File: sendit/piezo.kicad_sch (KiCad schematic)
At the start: 3 parts, among them Q4 AO3400A

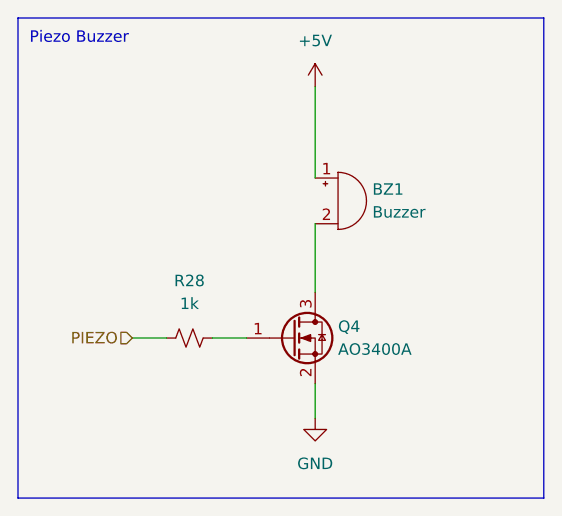
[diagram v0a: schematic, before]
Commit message: piezo resistor
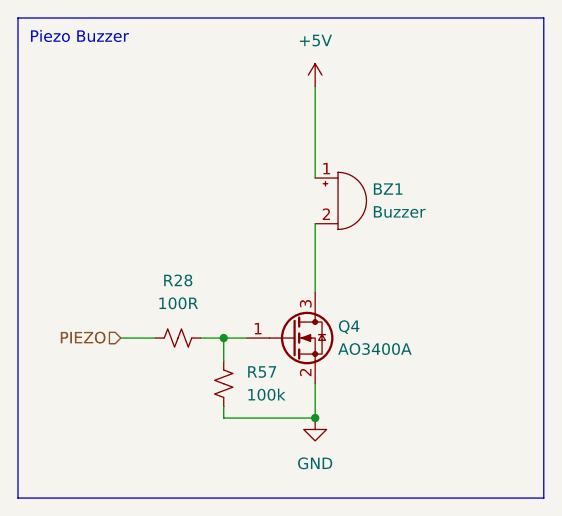
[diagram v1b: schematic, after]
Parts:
- added R57: 100k, Resistor_SMD:R_0603_1608Metric, symbol Device:R_Small_US
- R28: value 1k -> 100R; LCSC C95781 -> (none)
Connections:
- net GND: now also R57.2
- net at Q4.1 (G), R28.1: now also R57.1
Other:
- moved on the sheet: R28
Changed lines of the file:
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@@
 		)
+	)
+	(junction
+		(at 143.51 102.87)
+		(diameter 0)
+		(color 0 0 0 0)
+	)
+	(junction
+		(at 133.35 93.98)
+		(diameter 0)
+		(color 0 0 0 0)
 	)
 	(wire
@@
 	(wire
 		(pts
+			(xy 133.35 93.98) (xy 135.89 93.98)
+		)
+		(stroke
+			(width 0)
+			(type default)
+		)
+	)
+	(wire
+		(pts
+			(xy 133.35 93.98) (xy 133.35 96.52)
+		)
+		(stroke
+			(width 0)
+			(type default)
+		)
+	)
+	(wire
+		(pts
 			(xy 143.51 66.04) (xy 143.51 76.2)
 		)
@@
 	(wire
 		(pts
-			(xy 132.08 93.98) (xy 135.89 93.98)
+			(xy 130.81 93.98) (xy 133.35 93.98)
 		)
 		(stroke
@@
 	(wire
 		(pts
-			(xy 123.19 93.98) (xy 127 93.98)
+			(xy 133.35 101.6) (xy 133.35 102.87)
+		)
+		(stroke
+			(width 0)
+			(type default)
+		)
+	)
+	(wire
+		(pts
+			(xy 121.92 93.98) (xy 125.73 93.98)
+		)
+		(stroke
+			(width 0)
+			(type default)
+		)
+	)
+	(wire
+		(pts
+			(xy 133.35 102.87) (xy 143.51 102.87)
 		)
 		(stroke
@@
 	(hierarchical_label "PIEZO"
 		(shape input)
-		(at 123.19 93.98 180)
+		(at 121.92 93.98 180)
 		(effects
 			(font
@@
 	(symbol
 		(lib_id "Device:R_Small_US")
-		(at 129.54 93.98 270)
+		(at 128.27 93.98 270)
 		(unit 1)
 		(exclude_from_sim no)
@@
 		(fields_autoplaced yes)
 		(property "Reference" "R28"
-			(at 129.54 87.63 90)
-			(effects
-				(font
-					(size 1.27 1.27)
-				)
-			)
-		)
-		(property "Value" "1k"
-			(at 129.54 90.17 90)
+			(at 128.27 87.63 90)
+			(effects
+				(font
+					(size 1.27 1.27)
+				)
+			)
+		)
+		(property "Value" "100R"
+			(at 128.27 90.17 90)
 			(effects
 				(font
@@
 		)
 		(property "Footprint" "Resistor_SMD:R_0603_1608Metric"
-			(at 129.54 93.98 0)
+			(at 128.27 93.98 0)
 			(effects
 				(font
@@
 		)
 		(property "Datasheet" "~"
-			(at 129.54 93.98 0)
+			(at 128.27 93.98 0)
 			(effects
 				(font
@@
 		)
 		(property "Description" "Resistor, small US symbol"
-			(at 129.54 93.98 0)
-			(effects
-				(font
-					(size 1.27 1.27)
-				)
-				(hide yes)
-			)
-		)
-		(property "LCSC" "C95781"
-			(at 129.54 93.98 0)
-			(effects
-				(font
-					(size 1.27 1.27)
-				)
-				(hide yes)
-			)
-		)
-		(property "ALT" ""
-			(at 129.54 93.98 0)
+			(at 128.27 93.98 0)
 			(effects
 				(font
@@
 					(unit 1)
 				)
+			)
+		)
+	)
+	(symbol
+		(lib_id "Device:R_Small_US")
+		(at 133.35 99.06 0)
+		(unit 1)
+		(exclude_from_sim no)
+		(in_bom yes)
+		(on_board yes)
+		(dnp no)
+		(fields_autoplaced yes)
+		(property "Reference" "R57"
+			(at 135.89 97.7899 0)
+			(effects
+				(font
+					(size 1.27 1.27)
+				)
+				(justify left)
+			)
+		)
+		(property "Value" "100k"
+			(at 135.89 100.3299 0)
+			(effects
+				(font
+					(size 1.27 1.27)
+				)
+				(justify left)
+			)
+		)
+		(property "Footprint" "Resistor_SMD:R_0603_1608Metric"
+			(at 133.35 99.06 0)
+			(effects
+				(font
+					(size 1.27 1.27)
+				)
+				(hide yes)
+			)
+		)
+		(property "Datasheet" "~"
+			(at 133.35 99.06 0)
+			(effects
+				(font
+					(size 1.27 1.27)
+				)
+				(hide yes)
+			)
+		)
+		(property "Description" "Resistor, small US symbol"
+			(at 133.35 99.06 0)
+			(effects
+				(font
+					(size 1.27 1.27)
+				)
+				(hide yes)
+			)
+		)
+		(pin "1"
+		)
+		(pin "2"
+		)
+		(instances
+			(project "sendit"
+				(path "/a355e4d0-2918-44fc-be8d-2503b84c6d6c/730ddc54-308b-4950-8f3a-2beb2098c60b"
+					(reference "R57")
+					(unit 1)
+				)

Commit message: bom and placement looking good.
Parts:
- BZ1: Rotation Offset (none) -> 90
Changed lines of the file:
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@@
+			)
+		)
+		(property "LCSC Part Name" ""
+			(at 140.97 93.98 0)
+			(effects
+				(font
+					(size 1.27 1.27)
+				)
+				(hide yes)
+			)
+		)
+		(property "Manufacturer" ""
+			(at 140.97 93.98 0)
+			(effects
+				(font
+					(size 1.27 1.27)
+				)
+				(hide yes)
+			)
+		)
+		(property "Manufacturer Part" ""
+			(at 140.97 93.98 0)
+			(effects
+				(font
+					(size 1.27 1.27)
+				)
+				(hide yes)
+			)
+		)
+		(property "Supplier" ""
+			(at 140.97 93.98 0)
+			(effects
+				(font
+					(size 1.27 1.27)
+				)
+				(hide yes)
+			)
+		)
+		(property "Supplier Part" ""
+			(at 140.97 93.98 0)
+			(effects
+				(font
+					(size 1.27 1.27)
+				)
+				(hide yes)
 			)
 		)
@@
 			)
 		)
+		(property "LCSC Part Name" ""
+			(at 128.27 93.98 90)
+			(effects
+				(font
+					(size 1.27 1.27)
+				)
+				(hide yes)
+			)
+		)
+		(property "Manufacturer" ""
+			(at 128.27 93.98 90)
+			(effects
+				(font
+					(size 1.27 1.27)
+				)
+				(hide yes)
+			)
+		)
+		(property "Manufacturer Part" ""
+			(at 128.27 93.98 90)
+			(effects
+				(font
+					(size 1.27 1.27)
+				)
+				(hide yes)
+			)
+		)
+		(property "Supplier" ""
+			(at 128.27 93.98 90)
+			(effects
+				(font
+					(size 1.27 1.27)
+				)
+				(hide yes)
+			)
+		)
+		(property "Supplier Part" ""
+			(at 128.27 93.98 90)
+			(effects
+				(font
+					(size 1.27 1.27)
+				)
+				(hide yes)
+			)
+		)
 		(pin "1"
 		)
@@
 			)
 		)
+		(property "LCSC Part Name" ""
+			(at 133.35 99.06 0)
+			(effects
+				(font
+					(size 1.27 1.27)
+				)
+				(hide yes)
+			)
+		)
+		(property "Manufacturer" ""
+			(at 133.35 99.06 0)
+			(effects
+				(font
+					(size 1.27 1.27)
+				)
+				(hide yes)
+			)
+		)
+		(property "Manufacturer Part" ""
+			(at 133.35 99.06 0)
+			(effects
+				(font
+					(size 1.27 1.27)
+				)
+				(hide yes)
+			)
+		)
+		(property "Supplier" ""
+			(at 133.35 99.06 0)
+			(effects
+				(font
+					(size 1.27 1.27)
+				)
+				(hide yes)
+			)
+		)
+		(property "Supplier Part" ""
+			(at 133.35 99.06 0)
+			(effects
+				(font
+					(size 1.27 1.27)
+				)
+				(hide yes)
+			)
+		)
 		(pin "1"
 		)
@@
 			(at 146.05 78.74 0)
 			(effects
+				(font
+					(size 1.27 1.27)
+				)
+				(hide yes)
+			)
+		)
+		(property "Rotation Offset" "90"
+			(at 146.05 78.74 0)
+			(effects
